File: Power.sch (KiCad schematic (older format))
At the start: 24 parts, among them U13 L78L12_SOT89, U14 MP4560_QFN10, U3 L78L12_SOT89, U4 LP2985-3.3

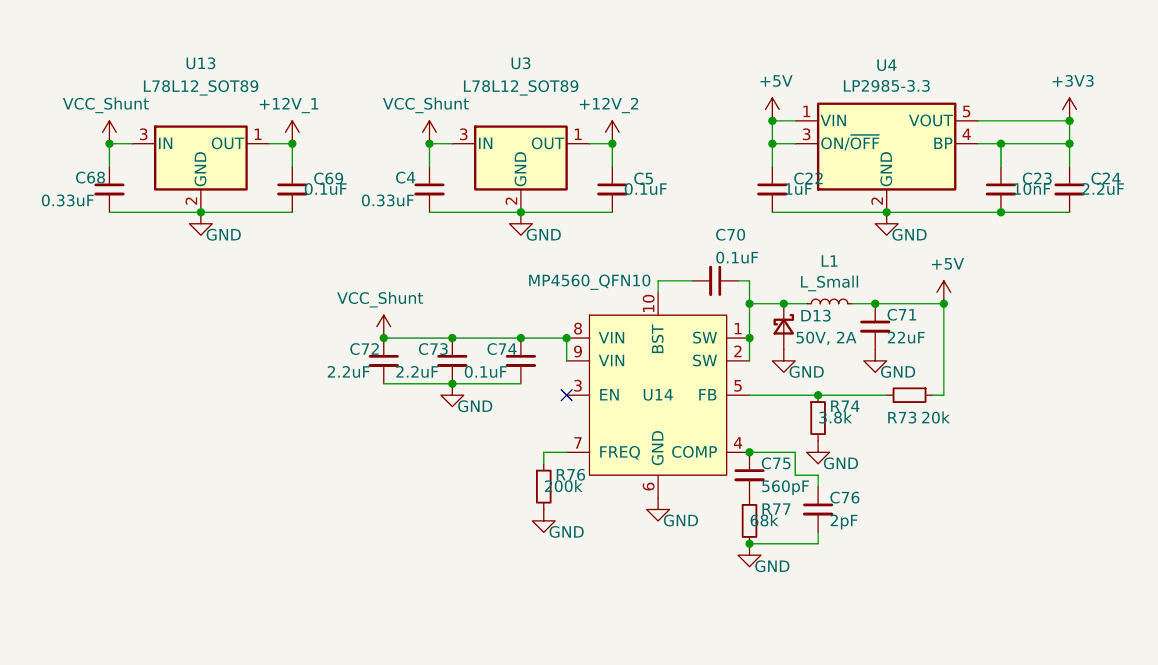
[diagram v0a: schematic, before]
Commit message: Added more PNGs
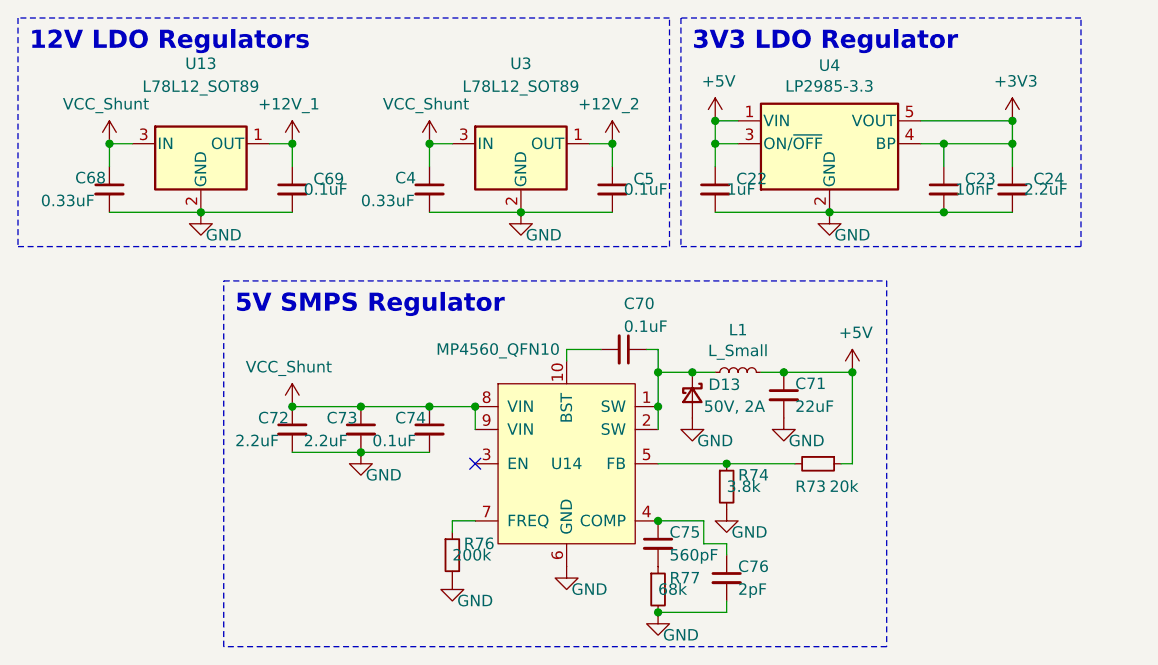
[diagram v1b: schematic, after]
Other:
- note added: "12V LDO Regulators"
- note added: "3V3 LDO Regulator"
- note added: "5V SMPS Regulator"
- moved on the sheet: C22, C23, C24, C70, C71, C72, C73, C74, C75, C76, D13, L1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
